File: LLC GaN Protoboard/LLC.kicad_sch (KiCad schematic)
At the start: 10 parts, among them IC1 FAN73912AMX, IC2 BZX84-C5V6,215, IC3 BZX84-C5V6,215, IC4 GAN7R0-150LBE, IC5 GAN7R0-150LBE, IC6 BZX84-C5V6,215

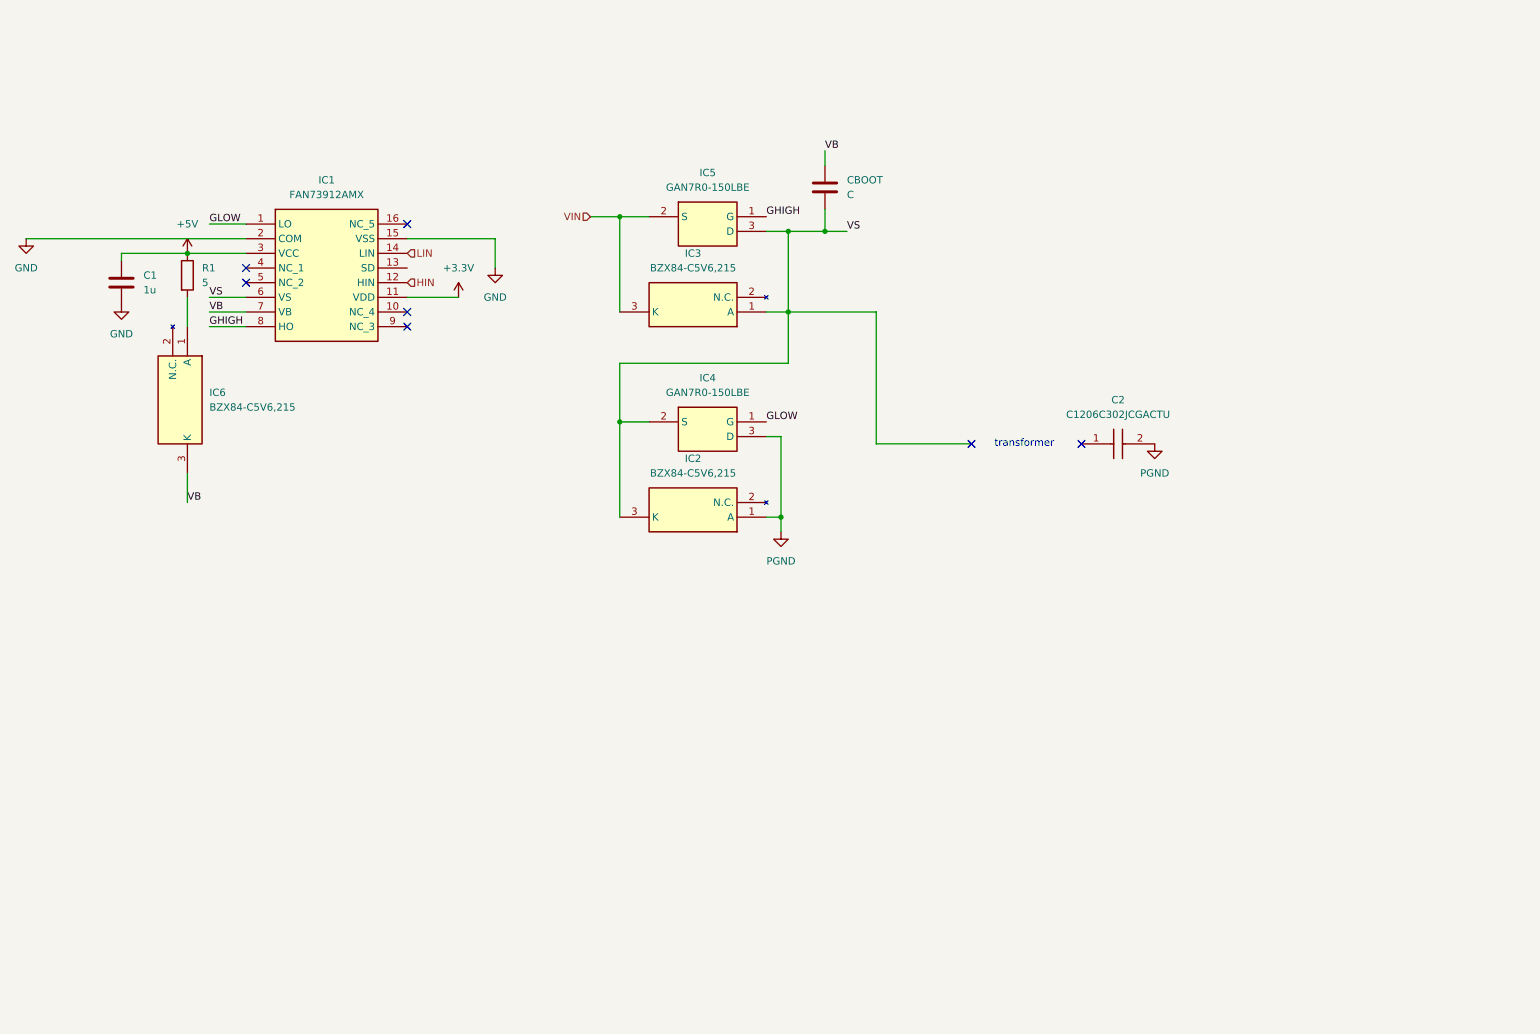
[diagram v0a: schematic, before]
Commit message: Initial layout
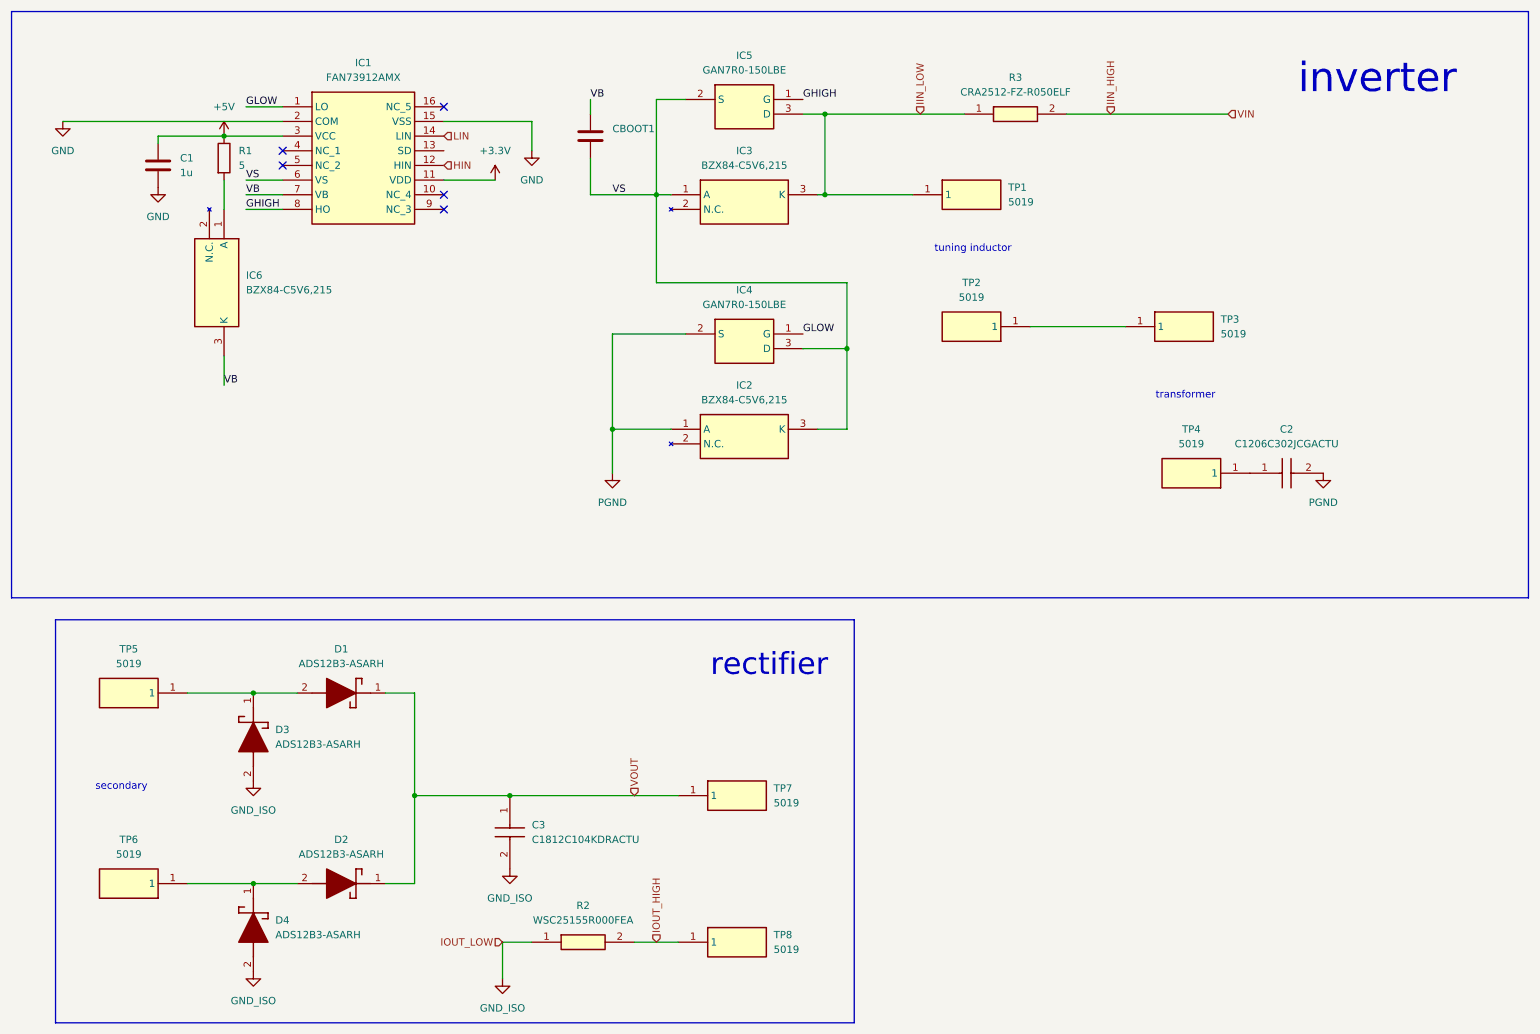
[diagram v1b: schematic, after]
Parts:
- removed CBOOT: C, symbol Device:C
- added C3: C1812C104KDRACTU, C1812C104KDRACTU:C1812, symbol C1812C104KDRACTU:C1812C104KDRACTU
- added CBOOT1: C, Capacitor_SMD:C_0603_1608Metric, symbol Device:C
- added D1, D2, D3, D4: ADS12B3-ASARH, ADS12B3-ASARH:ADS12B3ASARH, symbol ADS12B3-ASARH:ADS12B3-ASARH
- added R2: WSC25155R000FEA, WSC25155R000FEA:RESM6438X317N, symbol WSC25155R000FEA:WSC25155R000FEA
- added R3: CRA2512-FZ-R050ELF, CRA2512-FZ-R050ELF:RESC6434X90N, symbol CRA2512-FZ-R050ELF:CRA2512-FZ-R050ELF
- added TP1, TP2, TP3, TP4, TP5, TP6, TP7, TP8: 5019, 5019:5019, symbol 5019:5019
- C1: footprint (none) -> Capacitor_SMD:C_0603_1608Metric
- C2: footprint C1206 -> C1206C302JCGACTU:C1206
- IC1: footprint SOIC127P1032X264-16N -> FAN73912AMX:SOIC127P1032X264-16N
- IC2, IC3, IC6: footprint SOT95P230X110-3N -> BZX84-C5V6,215:SOT95P230X110-3N
- IC4, IC5: footprint GAN7R0150LBE -> GAN7R0-150LBE:GAN7R0150LBE
- R1: footprint (none) -> Resistor_SMD:R_2010_5025Metric
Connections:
- net PGND: now also IC4.2 (S); no longer IC4.3 (D)
- net VB: now also CBOOT1.1
- net VS: now also IC4.3 (D), IC5.2 (S), CBOOT1.2; no longer IC4.2 (S), IC5.3 (D)
- net at C2.1: now also TP4.1
- net VIN renamed IIN_LOW
- net IIN_LOW: now also IC5.3 (D), R3.1, TP1.1; no longer IC5.2 (S)
- new net: TP2.1, TP3.1
- new net: D1.2 (A), D3.1 (K), TP5.1
- new net: D2.2 (A), D4.1 (K), TP6.1
- new net GND_ISO: C3.2, D3.2 (A), D4.2 (A), R2.1
- new net IIN_HIGH: R3.2
- new net IOUT_HIGH: R2.2, TP8.1
- new net VOUT: C3.1, D1.1 (K), D2.1 (K), TP7.1
- no-connect marks 7 -> 5
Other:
- note added: "inverter"
- note added: "rectifier"
- note added: "secondary"
- note added: "tuning inductor"
- moved on the sheet: C1, C2, IC1, IC2, IC3, IC4, IC5, IC6, R1

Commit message: Edited layout
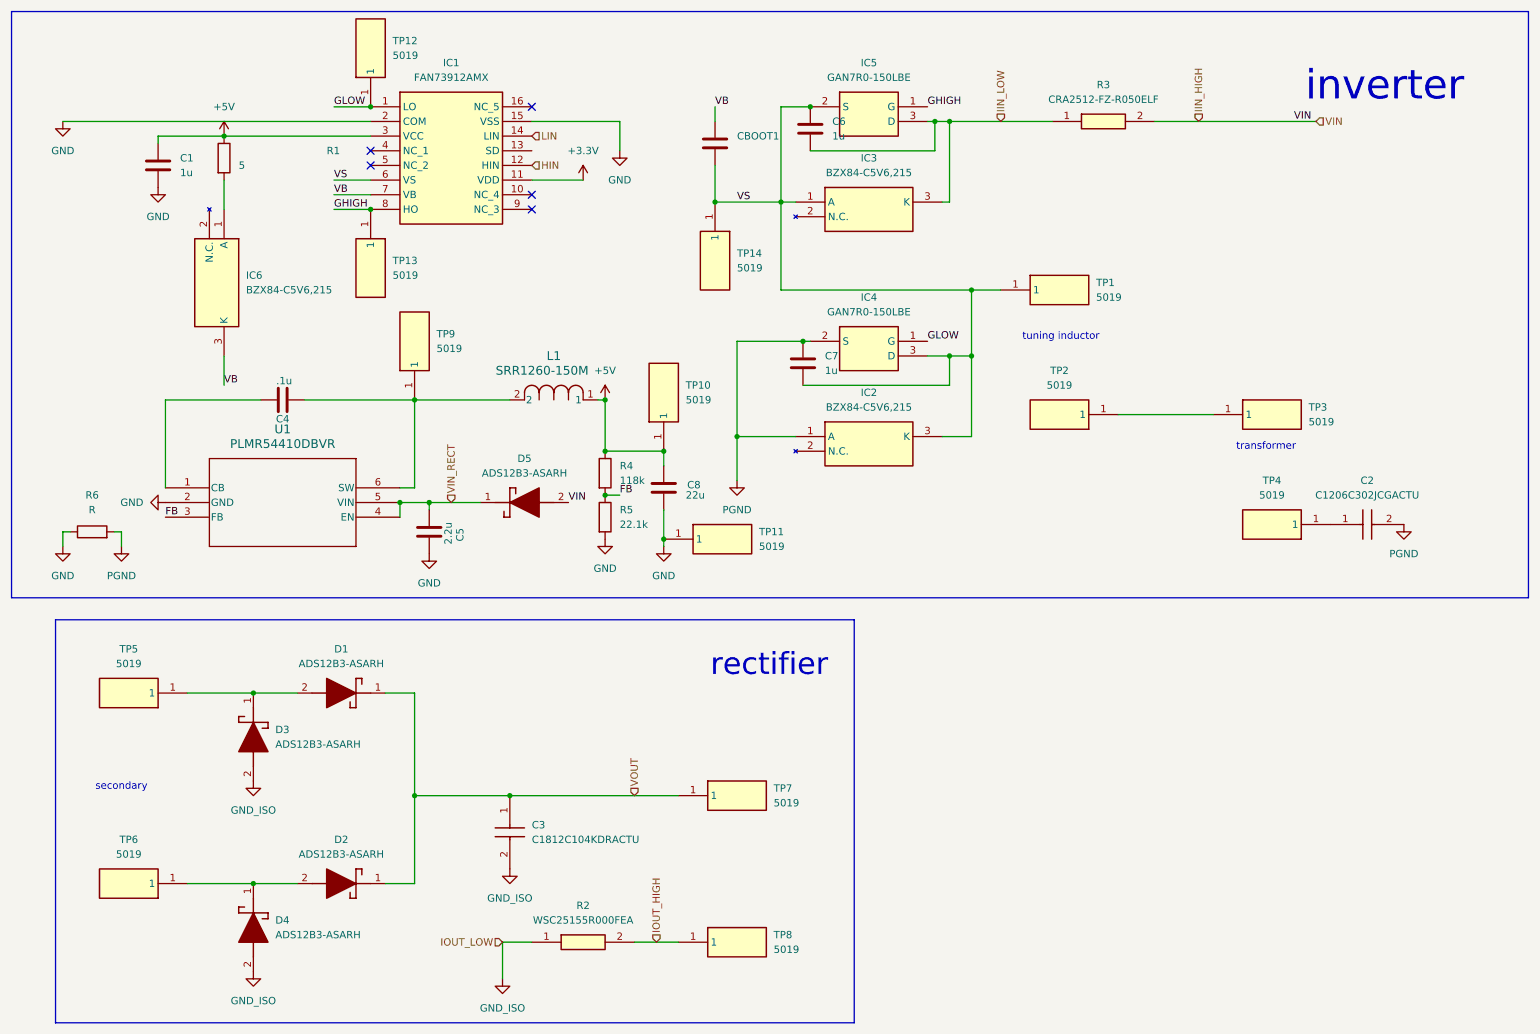
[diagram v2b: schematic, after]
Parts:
- added C4: .1u, Capacitor_SMD:C_0603_1608Metric, symbol Device:C
- added C5: 2.2u, Capacitor_SMD:C_0603_1608Metric, symbol Device:C
- added C6, C7: 1u, Capacitor_SMD:C_0603_1608Metric, symbol Device:C
- added C8: 22u, Capacitor_SMD:C_0603_1608Metric, symbol Device:C
- added D5: ADS12B3-ASARH, ADS12B3-ASARH:ADS12B3ASARH, symbol ADS12B3-ASARH:ADS12B3-ASARH
- added L1: SRR1260-150M, IND_BOURNS_SRR1260, symbol 2026-07-13_06-36-12:SRR1260-150M
- added R4: 118k, Resistor_SMD:R_2010_5025Metric, symbol Device:R
- added R5: 22.1k, Resistor_SMD:R_2010_5025Metric, symbol Device:R
- added R6: R, symbol Device:R
- added TP10, TP11, TP12, TP13, TP14, TP9: 5019, 5019:5019, symbol 5019:5019
- added U1: PLMR54410DBVR, U_SOT-23_TEX, symbol 2026-07-11_06-22-39:PLMR54410DBVR
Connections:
- net +5V: now also C8.1, L1.1, R4.1, TP10.1
- net GHIGH: now also TP13.1
- net GLOW: now also TP12.1
- net GND: now also C5.2, C8.2, R5.2, R6.1, TP11.1, U1.2 (GND)
- net IIN_HIGH: now also D5.2 (A)
- net IIN_LOW: now also C6.2; no longer TP1.1
- net PGND: now also C7.1, R6.2
- net VS: now also TP1.1, C6.1, C7.2, TP14.1
- new net: C4.2, L1.2, TP9.1, U1.6 (SW)
- new net: C4.1, U1.1 (CB)
- new net FB: R4.2, R5.1, U1.3 (FB)
- new net VIN_RECT: C5.1, D5.1 (K), U1.4 (EN), U1.5 (VIN)
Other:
- moved on the sheet: C2, CBOOT1, IC1, IC2, IC3, IC4, IC5, R3, TP1, TP2, TP3, TP4
